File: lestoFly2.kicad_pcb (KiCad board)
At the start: 2 copper layers, 35 x 40 mm, 43 parts, among them J1 Conn_01x02_Male, J10 Conn_01x07_Male, J2 Conn_01x06_Male, J3 Conn_Coaxial, J4 Micro_SD_Card_Det, J5 Conn_01x07_Male, J6 Conn_01x02_Male, J7 Conn_01x02_Male, J8 Conn_01x02_Male, J9 Conn_01x02_Male, Q1 DMN6140L, U1 NCP1117-1.8_TO252, U2 STM32H743ZITx, U3 ICM-20948, U4 ICM-20948, U5 RFM95W-868S2, U6 BMP280, Y1 25MHz

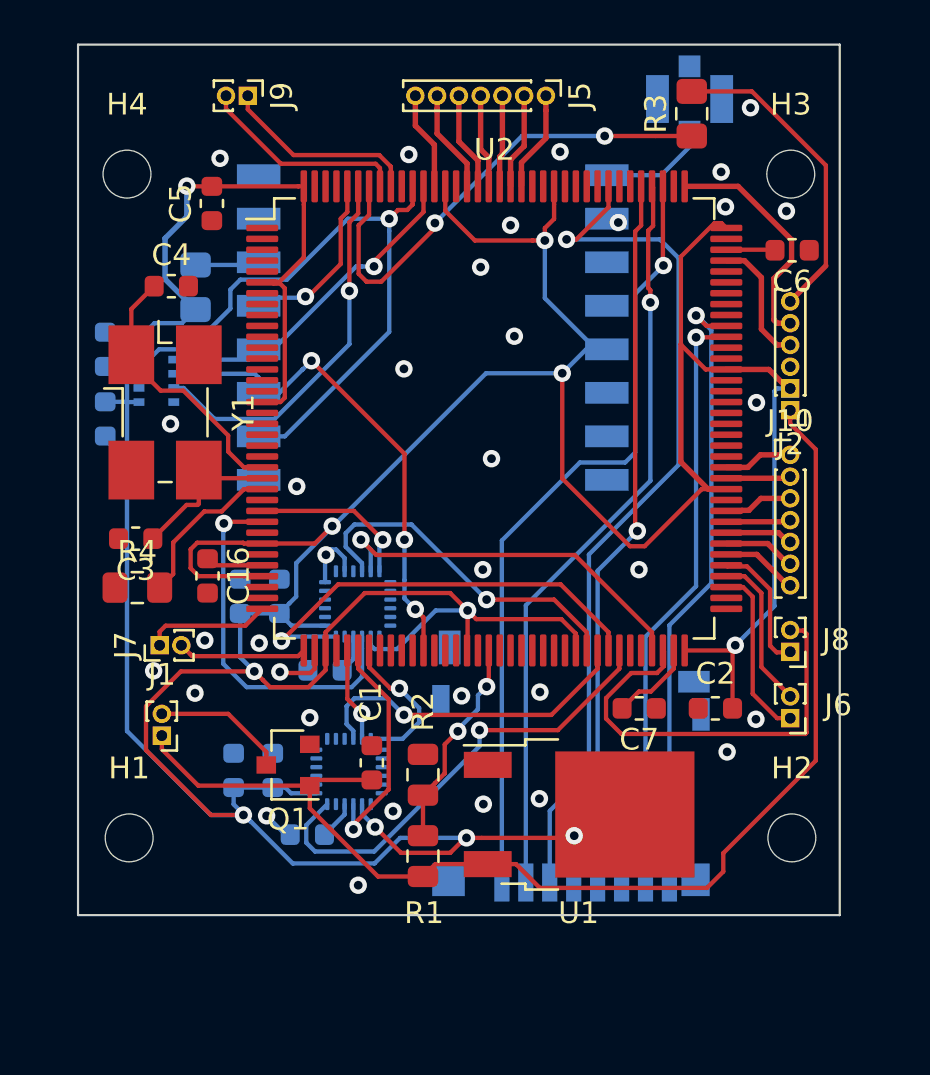
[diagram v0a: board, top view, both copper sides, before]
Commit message: varius fixes
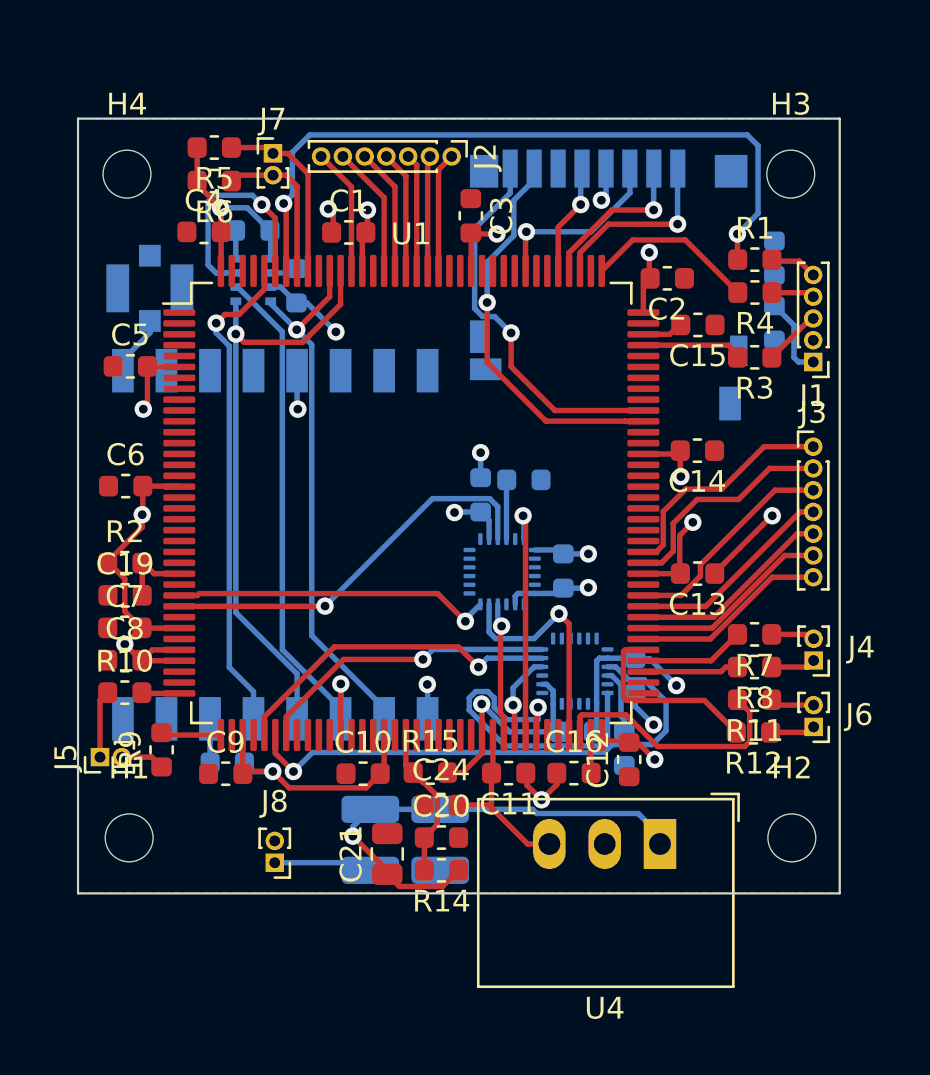
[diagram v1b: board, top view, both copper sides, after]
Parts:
- removed the C16 at (83.7, 89.5)
- removed the J2 at (110.5, 81.9)
- removed the J7 at (81.5, 92.7)
- removed Q1: DMN6140L, Package_TO_SOT_SMD:SOT-23
- removed Y1: 25MHz, Crystal:Crystal_SMD_0603-4Pin_6.0x3.5mm_HandSoldering
- added C1: 100nF, Capacitor_SMD:C_0603_1608Metric, F.Cu at (90.2, 73.7)
- added C14: 100nF, Capacitor_SMD:C_0603_1608Metric, F.Cu at (106.2, 83.8)
- added C19: 100nF, Capacitor_SMD:C_0603_1608Metric, F.Cu at (79.9, 90.4)
- added C2: 100nF, Capacitor_SMD:C_0603_1608Metric, F.Cu at (104.8, 75.8)
- added C20: 1nF, Capacitor_SMD:C_0603_1608Metric, F.Cu at (94.5, 101.5)
- added C22: 100nF, Capacitor_SMD:C_0603_1608Metric, B.Cu at (102.8, 97.4)
- added C23: 100nF, Capacitor_SMD:C_0603_1608Metric, B.Cu at (103.3, 94.1)
- added C25: 100nF, Capacitor_SMD:C_0603_1608Metric, B.Cu at (100.6, 96.7)
- added C26: 100nF, Capacitor_SMD:C_0603_1608Metric, B.Cu at (109.8, 74.9)
- added C27: 1uF, Capacitor_SMD:C_0603_1608Metric, B.Cu at (109.8, 77.9)
- added C28: 100nF, Capacitor_SMD:C_0603_1608Metric, B.Cu at (98.2, 85.1)
- added C29: 100nF, Capacitor_SMD:C_0603_1608Metric, B.Cu at (96.2, 85.8)
- added C30: 100nF, Capacitor_SMD:C_0603_1608Metric, B.Cu at (100.0, 89.3)
- added C6: 100nF, Capacitor_SMD:C_0603_1608Metric, F.Cu at (79.9, 85.4)
- added C7: 100nF, Capacitor_SMD:C_0603_1608Metric, F.Cu at (79.9, 91.9)
- added D1: D, Diode_SMD:D_1210_3225Metric, B.Cu at (94.4, 101.6)
- added F1: Polyfuse, Fuse:Fuse_1210_3225Metric, B.Cu at (91.2, 101.6)
- added J5: Conn_01x02_Male, Connector_PinHeader_1.00mm:PinHeader_1x02_P1.00mm_Vertical, F.Cu at (78.8, 97.8)
- added J8: Conn_01x02_Male, Connector_PinHeader_1.00mm:PinHeader_1x02_P1.00mm_Vertical, F.Cu at (86.8, 102.7)
- added R10: 47ohm, Resistor_SMD:R_0603_1608Metric, F.Cu at (79.9, 94.9)
- added R11: 47ohm, Resistor_SMD:R_0603_1608Metric, F.Cu at (108.8, 95.2)
- added R12: 47ohm, Resistor_SMD:R_0603_1608Metric, F.Cu at (108.8, 96.7)
- added R2: 10K, Resistor_SMD:R_0603_1608Metric, F.Cu at (79.9, 88.9)
- added R3: 47ohm, Resistor_SMD:R_0603_1608Metric, F.Cu at (108.8, 79.5)
- added R5: 1.5k, Resistor_SMD:R_0603_1608Metric, F.Cu at (84.0, 69.8)
- added R6: 1.5k, Resistor_SMD:R_0603_1608Metric, F.Cu at (84.0, 71.4)
- added R7: 47ohm, Resistor_SMD:R_0603_1608Metric, F.Cu at (108.8, 92.2)
- added R8: 47ohm, Resistor_SMD:R_0603_1608Metric, F.Cu at (108.8, 93.7)
- added R9: 47ohm, Resistor_SMD:R_0603_1608Metric, F.Cu at (81.6, 97.5)
- C10, C11, C12, C13, C8, C9: moved to F.Cu
- C21: renamed from C1; footprint Capacitor_SMD:C_0603_1608Metric -> Resistor_SMD:R_0805_2012Metric
- C3, C4: value 3.9pF -> 100nF
- J1: value Conn_01x02_Male -> Conn_01x05_Male; footprint Connector_PinHeader_1.00mm:PinHeader_1x02_P1.00mm_Vertical -> Connector_PinHeader_1.00mm:PinHeader_1x05_P1.00mm_Vertical
- R1: renamed from R3; footprint Resistor_SMD:R_0805_2012Metric_Pad1.15x1.40mm_HandSolder -> Resistor_SMD:R_0603_1608Metric
- R13: renamed from R5; footprint Resistor_SMD:R_0805_2012Metric_Pad1.15x1.40mm_HandSolder -> Resistor_SMD:R_0603_1608Metric
- R14: renamed from R1; footprint Resistor_SMD:R_0805_2012Metric -> Resistor_SMD:R_0603_1608Metric
- R15: renamed from R2; footprint Resistor_SMD:R_0805_2012Metric -> Resistor_SMD:R_0603_1608Metric
- R4: value 10K -> 47ohm; footprint Resistor_SMD:R_0805_2012Metric_Pad1.15x1.40mm_HandSolder -> Resistor_SMD:R_0603_1608Metric
- U1: value NCP1117-1.8_TO252 -> STM32H743ZITx; footprint Package_TO_SOT_SMD:TO-252-2 -> Package_QFP:LQFP-144_20x20mm_P0.5mm
- U2: value STM32H743ZITx -> RFM95W-868S2; footprint Package_QFP:LQFP-144_20x20mm_P0.5mm -> RF_Module:HOPERF_RFM9XW_SMD; moved to B.Cu
- U4: value ICM-20948 -> R-78C1.8-1.0; footprint Sensor_Motion:InvenSense_QFN-24_3x3mm_P0.4mm -> Converter_DCDC:Converter_DCDC_RECOM_R-78E-0.5_THT; moved to F.Cu
- U5: value RFM95W-868S2 -> ICM-20948; footprint RF_Module:HOPERF_RFM9XW_SMD -> Sensor_Motion:InvenSense_QFN-24_3x3mm_P0.4mm
- moved J1 34.5 mm to (111.5, 79.7)
- moved R4 31.5 mm to (108.9, 76.5), turned to 180 degrees
- moved J9 26.3 mm to (81.1, 76.3)
- moved J10 22.2 mm to (102.1, 76.1), turned to 0 degrees
- moved R13 21.9 mm to (84.6, 98.1), turned to 0 degrees
- moved C3 21.4 mm to (95.8, 73.0), turned to 270 degrees
- moved C13 21.0 mm to (106.2, 89.4), turned to 180 degrees
- moved C12 17.7 mm to (103.1, 98.0)
- moved U4 17.7 mm to (104.5, 101.8)
- moved U1 16.3 mm to (93.1, 86.2)
- moved C24 13.4 mm to (94.4, 100.0)
- moved U5 11.7 mm to (97.2, 89.3)
- moved U2 11.6 mm to (86.8, 88.1), turned to 90 degrees
- moved C8 11.6 mm to (79.9, 93.4), turned to 0 degrees
- moved U3 11.4 mm to (100.6, 93.9), turned to 270 degrees
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- renumbered C6 to C15, C7 to C16, C2 to C24, C14 to C31, C15 to C32, J4 to J10, J5 to J2, J10 to J3, J6 to J4, J8 to J6, J9 to J7, J3 to J9
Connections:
- C10 pad 1: +1V8 -> GND
- C10 pad 2: GND -> +1V8
- C11 pad 1: Net-(C11-Pad1) -> GND
- C11 pad 2: GND -> +1V8
- C12 pad 1: +1V8 -> GND
- C12 pad 2: GND -> +1V8
- C13 pad 1: +1V8 -> GND
- C13 pad 2: GND -> +1V8
- C3 pad 1: Net-(C3-Pad1) -> GND
- C3 pad 2: GND -> +1V8
- C4 pad 1: Net-(C4-Pad1) -> GND
- C4 pad 2: GND -> +1V8
- C8 pad 1: Net-(C8-Pad1) -> GND
- C8 pad 2: GND -> +1V8
- C9 pad 1: +1V8 -> GND
- C9 pad 2: GND -> +1V8
- J1 pad 1: VCC -> +1V8
- J1 pad 2: Net-(J1-Pad2) -> GND
- J2 pad 1: Net-(J5-Pad1) -> Net-(J2-Pad1)
- J2 pad 2: Net-(J5-Pad2) -> Net-(J2-Pad2)
- J2 pad 3: Net-(J5-Pad3) -> Net-(J2-Pad3)
- J2 pad 4: Net-(J5-Pad4) -> Net-(J2-Pad4)
- J2 pad 5: Net-(J5-Pad5) -> Net-(J2-Pad5)
- J2 pad 6: Net-(J5-Pad6) -> Net-(J2-Pad6)
- J2 pad 7: Net-(J5-Pad7) -> Net-(J2-Pad7)
- J3 pad 1: Net-(J10-Pad1) -> Net-(J3-Pad1)
- J3 pad 2: Net-(J10-Pad2) -> Net-(J3-Pad2)
- J3 pad 3: Net-(J10-Pad3) -> Net-(J3-Pad3)
- J3 pad 4: Net-(J10-Pad4) -> Net-(J3-Pad4)
- J3 pad 5: Net-(J10-Pad5) -> Net-(J3-Pad5)
- J3 pad 6: Net-(J10-Pad6) -> Net-(J3-Pad6)
- J3 pad 7: Net-(J10-Pad7) -> Net-(J3-Pad7)
- J4 pad 1: USART1_TX -> Net-(J4-Pad1)
- J4 pad 2: USART1_RX -> Net-(J4-Pad2)
- J6 pad 1: USART3_TX -> Net-(J6-Pad1)
- J6 pad 2: USART3_RX -> Net-(J6-Pad2)
- J9 pad 1: Net-(J3-Pad1) -> Net-(J9-Pad1)
- R1 pad 1: Net-(R3-Pad1) -> Net-(R1-Pad1)
- R1 pad 2: Net-(J2-Pad6) -> Net-(J1-Pad5)
- R13 pad 1: Net-(R5-Pad1) -> Net-(R13-Pad1)
- R4 pad 1: GND -> SWCLK
- U1 pad 1: GND -> Net-(U1-Pad1)
- U1 pad 2: +1V8 -> Net-(U1-Pad2)
- U1 pad 3: VCC -> Net-(U1-Pad3)
- U2 pad 1: Net-(U2-Pad1) -> GND
- U2 pad 10: Net-(U2-Pad10) -> GND
- U2 pad 13: Net-(U2-Pad13) -> +1V8
- U2 pad 16: GND -> Net-(U2-Pad16)
- U2 pad 2: Net-(U2-Pad2) -> SPI3_MISO
- U2 pad 3: Net-(U2-Pad3) -> SPI3_MOSI
- U2 pad 4: Net-(U2-Pad4) -> SPI3_CLK
- U2 pad 5: Net-(U2-Pad5) -> CS_LORA
- U2 pad 6: +1V8 -> Net-(R13-Pad1)
- U2 pad 8: Net-(U2-Pad8) -> GND
- U2 pad 9: Net-(U2-Pad9) -> Net-(J9-Pad1)
- U3 pad 10: Net-(C8-Pad1) -> Net-(C22-Pad1)
- U4 pad 1: Net-(U4-Pad1) -> VCC
- U4 pad 2: Net-(U4-Pad2) -> GND
- U4 pad 3: Net-(U4-Pad3) -> +1V8
- U5 pad 1: GND -> Net-(U5-Pad1)
- U5 pad 10: GND -> Net-(C28-Pad1)
- U5 pad 12: Net-(U5-Pad12) -> INT_IMU2
- U5 pad 2: SPI3_MISO -> Net-(U5-Pad2)
- U5 pad 3: SPI3_MOSI -> Net-(U5-Pad3)
- U5 pad 4: SPI3_CLK -> Net-(U5-Pad4)
- U5 pad 5: CS_LORA -> Net-(U5-Pad5)
- U5 pad 6: Net-(R5-Pad1) -> Net-(U5-Pad6)
- U5 pad 8: GND -> +1V8
- U5 pad 9: Net-(J3-Pad1) -> SPI2_MISO
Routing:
- net +1V8: track 239.6 -> 94.7 mm, vias 11 -> 17
- net VCC: track 56.9 -> 22.0 mm, vias 0 -> 1
- net Net-(R1-Pad1): track 0.00 -> 33.3 mm, vias 0 -> 2
- net SDMMC1_CMD: track 40.1 -> 8.43 mm
- net SDMMC1_D2: track 36.3 -> 8.43 mm
- net SDMMC1_CK: track 32.9 -> 5.16 mm
- net SDMMC1_D3: track 34.5 -> 7.44 mm
- net GND: track 6.70 -> 30.1 mm, vias 34 -> 8
- net Net-(R3-Pad1): track 22.6 -> 0.00 mm, vias 2 -> 0
- net CS_LORA: track 7.95 -> 22.6 mm
- net SPI1_MISO: track 10.6 -> 24.6 mm
- net Net-(C4-Pad1): track 12.4 -> 0.00 mm
- net SPI3_CLK: track 16.1 -> 27.6 mm
- net CS_IMU1: track 15.4 -> 3.94 mm
- net SPI1_CLK: track 4.34 -> 15.5 mm
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- added copper zone on In1.Cu, net +1V8
- added copper zone on In2.Cu, net GND
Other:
- board size 35 x 40 mm -> 35 x 35.6 mm
- copper layers 2 -> 4
